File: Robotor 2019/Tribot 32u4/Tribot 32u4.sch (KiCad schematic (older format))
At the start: 81 parts, among them J1 Conn_01x03_Male, J10 Conn_01x04, J11 Conn_01x04, J2 Conn_01x01, J3 USB_B_Mini, J4 Conn_01x04_Female, J5 Conn_01x04_Female, J6 AVR-ISP-6, J7 Conn_01x03_Female, J8 Conn_01x03_Female, J9 Conn_01x01, M1 Motor_DC, M2 Motor_DC, SW1 SW_Push, SW2 SW_Push, SW3 SW_Push, U3 AMS1117-5.0, U4 ATMEGA32U4-AU, U5 ITR8307, U6 L298P, U7 ITR8307, U8 ITR8307, U9 ITR8307, Y2 8Mhz

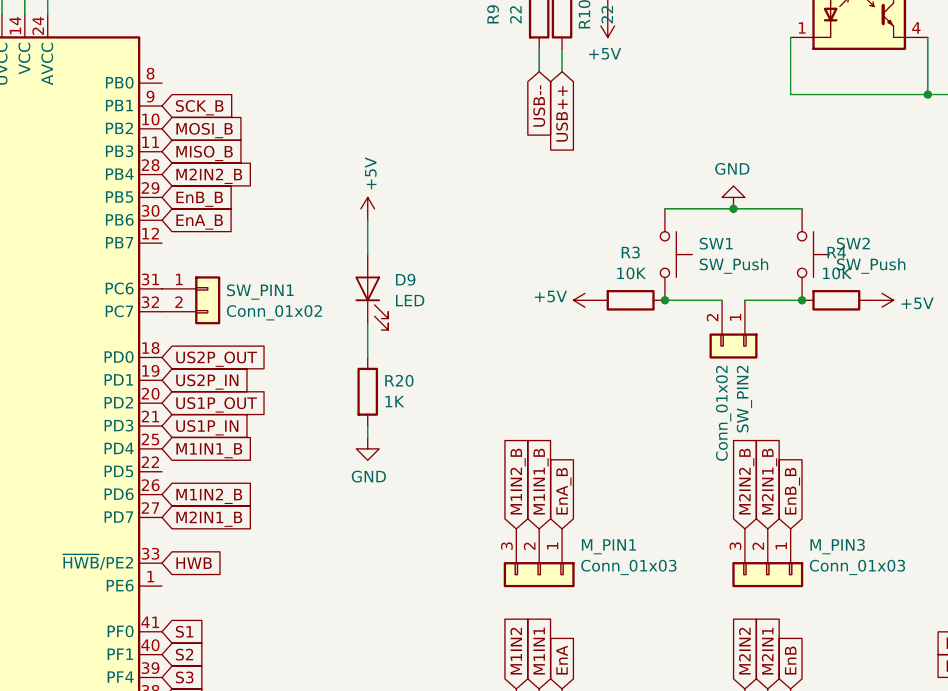
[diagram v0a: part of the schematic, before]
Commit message: Honestly I don't even remember
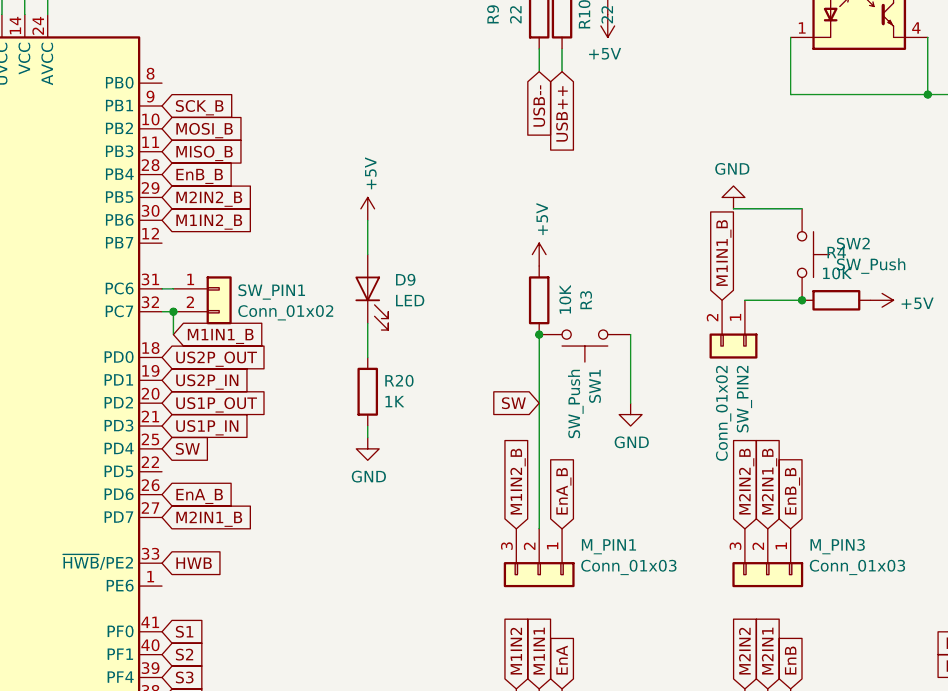
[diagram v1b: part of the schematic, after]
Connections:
- net EnA_B: now also U4.26 (PD6); no longer U4.30 (PB6)
- net EnB_B: now also U4.28 (PB4); no longer U4.29 (PB5)
- net M1IN1_B: now also SW_PIN1.2 (Pin_2), SW_PIN2.2 (Pin_2), U4.32 (PC7); no longer M_PIN1.2 (Pin_2), U4.25 (PD4)
- net M1IN2_B: now also U4.30 (PB6); no longer U4.26 (PD6)
- net M2IN2_B: now also U4.29 (PB5); no longer U4.28 (PB4)
- net SW: now reaches R3.1, SW1.2
- net SW: now also M_PIN1.2 (Pin_2), U4.25 (PD4); no longer SW_PIN2.2 (Pin_2)
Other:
- moved on the sheet: R3, SW1, SW_PIN1
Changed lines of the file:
@@
 Text GLabel 6850 4000 1    50   Input ~ 0
 M2IN1_B
-Text GLabel 5850 4000 1    50   Input ~ 0
+Text GLabel 4250 3150 2    50   Input ~ 0
 M1IN1_B
 Text GLabel 5750 4000 1    50   Input ~ 0
@@
 $EndComp
 $Comp
-L Switch:SW_Push SW1
-U 1 1 5D4D1350
-P 6400 2800
-F 0 "SW1" V 6354 2948 50  0000 L CNN
-F 1 "SW_Push" V 6445 2948 50  0000 L CNN
-F 2 "Button_Switch_SMD:SW_SPST_EVQPE1" H 6400 3000 50  0001 C CNN
-F 3 "~" H 6400 3000 50  0001 C CNN
-	1    6400 2800
-	0    1    1    0
-$EndComp
-Wire Wire Line
-	6400 2600 6700 2600
-$Comp
 L power:GND #PWR0113
 U 1 1 5D4E8556
@@
 	-1   0    0    1
 $EndComp
-Connection ~ 6700 2600
 Wire Wire Line
 	6700 2600 7000 2600
@@
 	0    1    1    0
 $EndComp
-Wire Wire Line
-	6400 3000 6650 3000
 Wire Wire Line
 	7000 3000 6750 3000
@@
 	-1   0    0    1
 $EndComp
-Text GLabel 4200 2650 2    50   Input ~ 0
-EnA_B
-Text GLabel 4200 2550 2    50   Input ~ 0
+Text GLabel 4200 2450 2    50   Input ~ 0
 EnB_B
-Text GLabel 4200 3650 2    50   Input ~ 0
+Text GLabel 6650 3000 1    50   Input ~ 0
 M1IN1_B
-Text GLabel 4200 3850 2    50   Input ~ 0
-M1IN2_B
-Text GLabel 4200 3950 2    50   Input ~ 0
-M2IN1_B
 $Comp
 L Connector_Generic:Conn_01x02 SW_PIN1
 U 1 1 5D505287
-P 4400 2950
-F 0 "SW_PIN1" H 4480 2942 50  0000 L CNN
-F 1 "Conn_01x02" H 4480 2851 50  0000 L CNN
-F 2 "Connector_PinSocket_2.54mm:PinSocket_1x02_P2.54mm_Vertical" H 4400 2950 50  0001 C CNN
-F 3 "~" H 4400 2950 50  0001 C CNN
-	1    4400 2950
+P 4450 2950
+F 0 "SW_PIN1" H 4530 2942 50  0000 L CNN
+F 1 "Conn_01x02" H 4530 2851 50  0000 L CNN
+F 2 "Connector_PinSocket_2.54mm:PinSocket_1x02_P2.54mm_Vertical" H 4450 2950 50  0001 C CNN
+F 3 "~" H 4450 2950 50  0001 C CNN
+	1    4450 2950
 	1    0    0    -1
 $EndComp
@@
 Text GLabel 4200 4750 2    50   Input ~ 0
 S4
-Text GLabel 4200 2450 2    50   Input ~ 0
+Text GLabel 4200 2550 2    50   Input ~ 0
 M2IN2_B
 Text GLabel 4200 4850 2    50   Input ~ 0
@@
 $EndComp
 $Comp
-L Device:R R3
-U 1 1 5D5E9CA7
-P 6250 3000
-F 0 "R3" V 6043 3000 50  0000 C CNN
-F 1 "10K" V 6134 3000 50  0000 C CNN
-F 2 "Resistor_SMD:R_0805_2012Metric_Pad1.15x1.40mm_HandSolder" V 6180 3000 50  0001 C CNN
-F 3 "~" H 6250 3000 50  0001 C CNN
-	1    6250 3000
-	0    1    1    0
-$EndComp
-Connection ~ 6400 3000
-$Comp
 L Device:R R4
 U 1 1 5D5EABDC
@@
 	1    7300 3000
 	0    1    1    0
-$EndComp
-$Comp
-L power:+5V #PWR0124
-U 1 1 5D5EB490
-P 6100 3000
-F 0 "#PWR0124" H 6100 2850 50  0001 C CNN
-F 1 "+5V" V 6115 3128 50  0000 L CNN
-F 2 "" H 6100 3000 50  0001 C CNN
-F 3 "" H 6100 3000 50  0001 C CNN
-	1    6100 3000
-	0    -1   -1   0
 $EndComp
 Text GLabel 3000 2850 0    50   Input ~ 0
@@
 	0    -1   -1   0
 $EndComp
+Text GLabel 4200 3950 2    50   Input ~ 0
+M2IN1_B
+Text GLabel 4200 3850 2    50   Input ~ 0
+EnA_B
+Text GLabel 4200 2650 2    50   Input ~ 0
+M1IN2_B
+Wire Wire Line
+	4250 3150 4250 3050
+Wire Wire Line
+	4250 3050 4200 3050
+Connection ~ 4250 3050
+Wire Wire Line
+	4250 2950 4200 2950
+$Comp
+L power:+5V #PWR0124
+U 1 1 5D5EB490
+P 5850 2850
+F 0 "#PWR0124" H 5850 2700 50  0001 C CNN
+F 1 "+5V" V 5865 2978 50  0000 L CNN
+F 2 "" H 5850 2850 50  0001 C CNN
+F 3 "" H 5850 2850 50  0001 C CNN
+	1    5850 2850
+	1    0    0    -1
+$EndComp
+Connection ~ 5850 3150
+$Comp
+L Device:R R3
+U 1 1 5D5E9CA7
+P 5850 3000
+F 0 "R3" V 5643 3000 50  0000 C CNN
+F 1 "10K" V 5734 3000 50  0000 C CNN
+F 2 "Resistor_SMD:R_0805_2012Metric_Pad1.15x1.40mm_HandSolder" V 5780 3000 50  0001 C CNN
+F 3 "~" H 5850 3000 50  0001 C CNN
+	1    5850 3000
+	-1   0    0    1
+$EndComp
+Wire Wire Line
+	6250 3150 6250 3450
+$Comp
+L Switch:SW_Push SW1
+U 1 1 5D4D1350
+P 6050 3150
+F 0 "SW1" V 6004 3298 50  0000 L CNN
+F 1 "SW_Push" V 6095 3298 50  0000 L CNN
+F 2 "Button_Switch_SMD:SW_SPST_EVQPE1" H 6050 3350 50  0001 C CNN
+F 3 "~" H 6050 3350 50  0001 C CNN
+	1    6050 3150
+	-1   0    0    1
+$EndComp
+Wire Wire Line
+	5850 3150 5850 4000
+$Comp
+L power:GND #PWR?
+U 1 1 5D6F66DA
+P 6250 3450
+F 0 "#PWR?" H 6250 3200 50  0001 C CNN
+F 1 "GND" H 6255 3277 50  0000 C CNN
+F 2 "" H 6250 3450 50  0001 C CNN
+F 3 "" H 6250 3450 50  0001 C CNN
+	1    6250 3450
+	1    0    0    -1
+$EndComp
+Text GLabel 4200 3650 2    50   Input ~ 0
+SW
+Text GLabel 5850 3450 0    50   Input ~ 0
+SW
 $EndSCHEMATC
